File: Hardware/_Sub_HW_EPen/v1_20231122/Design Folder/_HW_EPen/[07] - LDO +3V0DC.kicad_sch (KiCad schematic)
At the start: 6 parts, among them U701 MIC5365-3.0YC5-TR

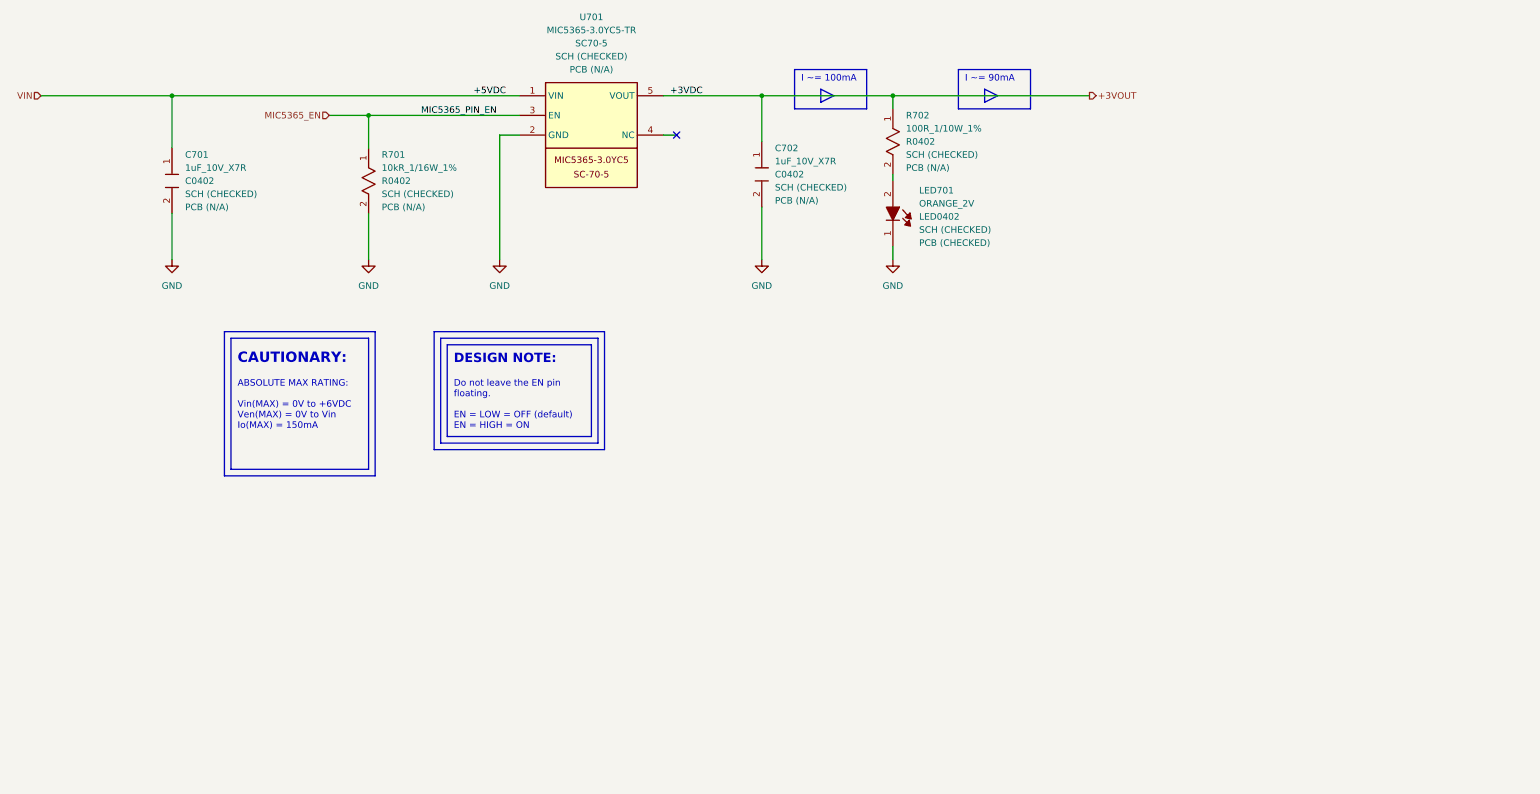
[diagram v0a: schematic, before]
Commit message: Updating file templates and structures...
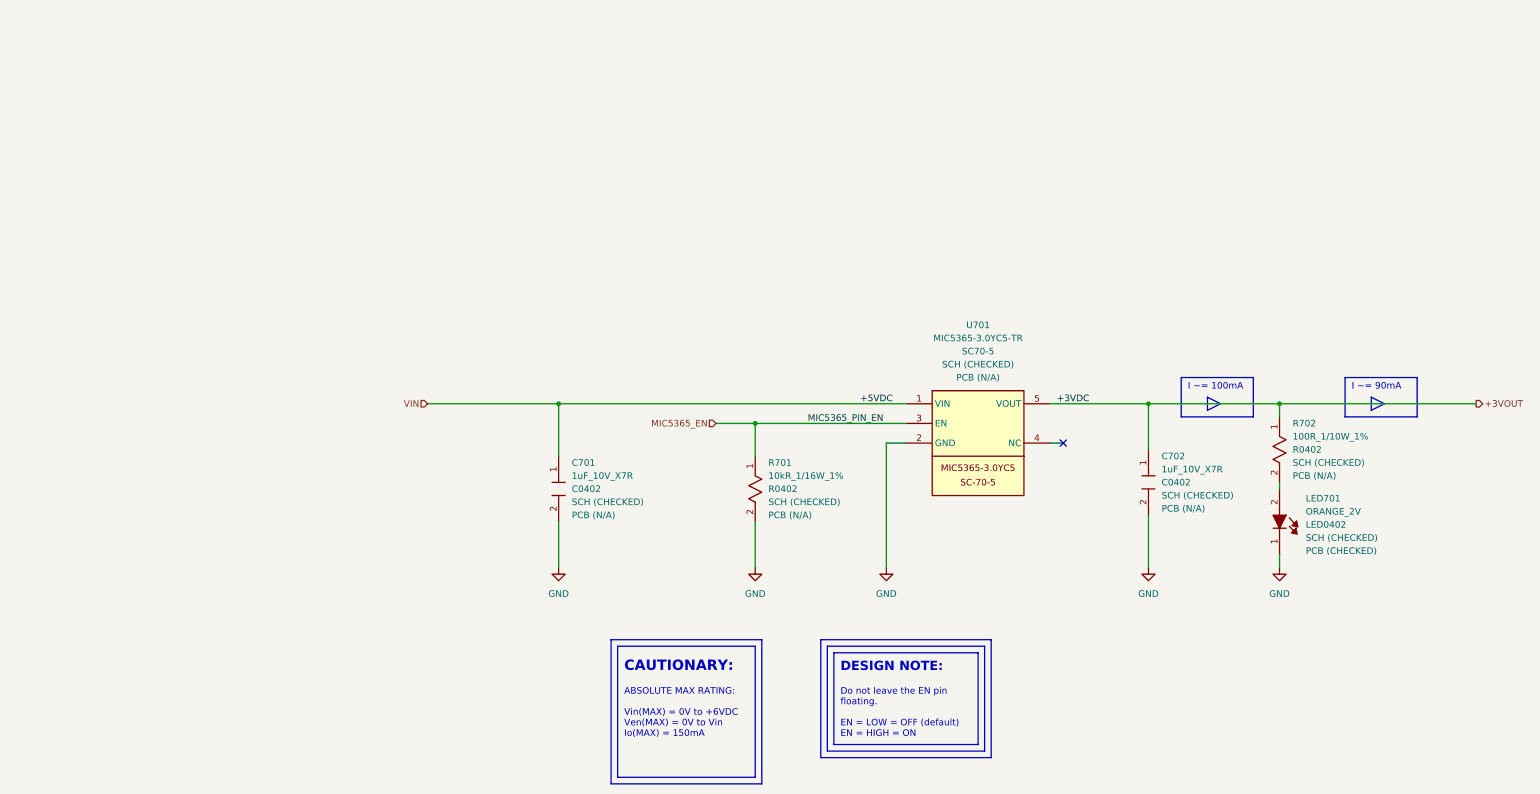
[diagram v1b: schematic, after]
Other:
- moved on the sheet: C701, C702, LED701, R701, R702, U701

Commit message: Updating Hardware File structures
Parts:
- C701, C702: Manufacturer (none) -> Murata Electronics; Part Number GRM155Z71A105KE01D -> (none); Part Number (Manufacturer) (none) -> GRM155Z71A105KE01D; Part Number (Vendor) (none) -> 490-GRM155Z71A105KE01DTR-ND; Vendor (none) -> Digikey
- LED701: Manufacturer (none) -> Harvatek Corporation; Part Number B2841UD--20D000614U1930 -> (none); Part Number (Manufacturer) (none) -> B2841UD--20D000614U1930; Part Number (Vendor) (none) -> 3147-B2841UD--20D000614U1930TR-ND; Vendor (none) -> Digikey
- R701: Manufacturer (none) -> Bourns Inc.; Part Number CR0402-FX-1002GLF -> (none); Part Number (Manufacturer) (none) -> CR0402-FX-1002GLF; Part Number (Vendor) (none) -> CR0402-FX-1002GLFTR-ND; Vendor (none) -> Digikey
- R702: Manufacturer (none) -> KOA Speer Electronics, Inc.; Part Number RK73H1ETTP1000F -> (none); Part Number (Manufacturer) (none) -> RK73H1ETTP1000F; Part Number (Vendor) (none) -> 2019-RK73H1ETTP1000FTR-ND; Vendor (none) -> Digikey
- U701: Manufacturer (none) -> Microchip Technology; Part Number MIC5365-3.0YC5-TR -> (none); Part Number (Manufacturer) (none) -> MIC5365-3.0YC5-TR; Part Number (Vendor) (none) -> 576-3191-2-ND; Vendor (none) -> Digikey
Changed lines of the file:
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@@
   (title_block
     (title "_HW_EPen")
-    (date "2023-11-28")
+    (date "2023/11/28")
     (rev "v1.0")
     (company "mend0z0")
     (comment 1 "v1.0")
     (comment 2 "CHECKED")
-    (comment 4 "_BOM_EPen.html")
-    (comment 5 "_HW_EPen.pcb")
+    (comment 3 "Siavash Taher Parvar")
+    (comment 4 "_BOM_EPen.csv")
+    (comment 5 "_HW_EPen.kicad_pcb")
     (comment 6 "_GBR_EPen.zip")
     (comment 7 "_BOM_EPen.html")
@@
       (effects (font (size 1.27 1.27)) (justify left) hide)
     )
-    (property "Part Number" "GRM155Z71A105KE01D" (at 220.98 191.77 0)
-      (effects (font (size 1.27 1.27)) (justify left) hide)
-    )
     (property "Link" "https://www.digikey.ca/en/products/detail/murata-electronics/GRM155Z71A105KE01D/13905035" (at 213.36 191.77 0)
       (effects (font (size 1.27 1.27)) (justify left) hide)
@@
       (effects (font (size 1.27 1.27)) (justify left))
     )
+    (property "Part Number (Vendor)" "490-GRM155Z71A105KE01DTR-ND" (at 201.93 189.23 0)
+      (effects (font (size 1.27 1.27)) hide)
+    )
+    (property "Part Number (Manufacturer)" "GRM155Z71A105KE01D" (at 223.52 191.77 0)
+      (effects (font (size 1.27 1.27)) (justify left) hide)
+    )
+    (property "Manufacturer" "Murata Electronics" (at 226.06 191.77 0)
+      (effects (font (size 1.27 1.27)) (justify left) hide)
+    )
+    (property "Vendor" "Digikey" (at 228.6 191.77 0)
+      (effects (font (size 1.27 1.27)) (justify left) hide)
+    )
     (pin "2")
     (pin "1")
@@
       (effects (font (size 1.27 1.27)) (justify left) hide)
     )
-    (property "Part Number" "RK73H1ETTP1000F" (at 360.68 184.15 0)
-      (effects (font (size 1.27 1.27)) (justify left) hide)
-    )
     (property "Link" "https://www.digikey.ca/en/products/detail/koa-speer-electronics-inc/RK73H1ETTP1000F/9844157" (at 353.06 184.15 0)
       (effects (font (size 1.27 1.27)) (justify left) hide)
@@
       (effects (font (size 1.27 1.27)) (justify left))
     )
+    (property "Part Number (Vendor)" "2019-RK73H1ETTP1000FTR-ND" (at 341.63 181.61 0)
+      (effects (font (size 1.27 1.27)) hide)
+    )
+    (property "Part Number (Manufacturer)" "RK73H1ETTP1000F" (at 363.22 184.15 0)
+      (effects (font (size 1.27 1.27)) (justify left) hide)
+    )
+    (property "Manufacturer" "KOA Speer Electronics, Inc." (at 365.76 184.15 0)
+      (effects (font (size 1.27 1.27)) (justify left) hide)
+    )
+    (property "Vendor" "Digikey" (at 368.3 184.15 0)
+      (effects (font (size 1.27 1.27)) (justify left) hide)
+    )
     (pin "1")
     (pin "2")
@@
       (effects (font (size 1.27 1.27)) (justify left) hide)
     )
-    (property "Part Number" "CR0402-FX-1002GLF" (at 259.08 191.77 0)
-      (effects (font (size 1.27 1.27)) (justify left) hide)
-    )
     (property "Link" "https://www.digikey.ca/en/products/detail/bourns-inc/CR0402-FX-1002GLF/3593192" (at 251.46 191.77 0)
       (effects (font (size 1.27 1.27)) (justify left) hide)
@@
       (effects (font (size 1.27 1.27)) (justify left))
     )
+    (property "Part Number (Vendor)" "CR0402-FX-1002GLFTR-ND" (at 240.03 189.23 0)
+      (effects (font (size 1.27 1.27)) hide)
+    )
+    (property "Part Number (Manufacturer)" "CR0402-FX-1002GLF" (at 261.62 191.77 0)
+      (effects (font (size 1.27 1.27)) (justify left) hide)
+    )
+    (property "Manufacturer" "Bourns Inc." (at 264.16 191.77 0)
+      (effects (font (size 1.27 1.27)) (justify left) hide)
+    )
+    (property "Vendor" "Digikey" (at 266.7 191.77 0)
+      (effects (font (size 1.27 1.27)) (justify left) hide)
+    )
     (pin "1")
     (pin "2")
@@
       (effects (font (size 1.27 1.27)) (justify left) hide)
     )
-    (property "Part Number" "B2841UD--20D000614U1930" (at 363.22 200.66 0)
-      (effects (font (size 1.27 1.27)) (justify left) hide)
-    )
     (property "Link" "https://www.digikey.ca/en/products/detail/harvatek-corporation/B2841UD-20D000614U1930/16729512" (at 355.6 200.66 0)
       (effects (font (size 1.27 1.27)) (justify left) hide)
@@
       (effects (font (size 1.27 1.27)) (justify left))
     )
+    (property "Part Number (Vendor)" "3147-B2841UD--20D000614U1930TR-ND" (at 341.63 195.58 0)
+      (effects (font (size 1.27 1.27)) hide)
+    )
+    (property "Part Number (Manufacturer)" "B2841UD--20D000614U1930" (at 365.76 200.66 0)
+      (effects (font (size 1.27 1.27)) (justify left) hide)
+    )
+    (property "Manufacturer" "Harvatek Corporation" (at 368.3 200.66 0)
+      (effects (font (size 1.27 1.27)) (justify left) hide)
+    )
+    (property "Vendor" "Digikey" (at 370.84 200.66 0)
+      (effects (font (size 1.27 1.27)) (justify left) hide)
+    )
     (pin "2")
     (pin "1")
@@
       (effects (font (size 1.27 1.27)) (justify left) hide)
     )
-    (property "Part Number" "GRM155Z71A105KE01D" (at 335.28 190.5 0)
-      (effects (font (size 1.27 1.27)) (justify left) hide)
-    )
     (property "Link" "https://www.digikey.ca/en/products/detail/murata-electronics/GRM155Z71A105KE01D/13905035" (at 327.66 190.5 0)
       (effects (font (size 1.27 1.27)) (justify left) hide)
@@
       (effects (font (size 1.27 1.27)) (justify left))
     )
+    (property "Part Number (Vendor)" "490-GRM155Z71A105KE01DTR-ND" (at 316.23 187.96 0)
+      (effects (font (size 1.27 1.27)) hide)
+    )
+    (property "Part Number (Manufacturer)" "GRM155Z71A105KE01D" (at 337.82 190.5 0)
+      (effects (font (size 1.27 1.27)) (justify left) hide)
+    )
+    (property "Manufacturer" "Murata Electronics" (at 340.36 190.5 0)
+      (effects (font (size 1.27 1.27)) (justify left) hide)
+    )
+    (property "Vendor" "Digikey" (at 342.9 190.5 0)
+      (effects (font (size 1.27 1.27)) (justify left) hide)
+    )
     (pin "2")
     (pin "1")
@@
       (effects (font (size 1.27 1.27)) (justify left) hide)
     )
-    (property "Part Number" "MIC5365-3.0YC5-TR" (at 276.86 157.48 0)
-      (effects (font (size 1.27 1.27)) (justify left) hide)
-    )
     (property "Link" "https://www.digikey.ca/en/products/detail/microchip-technology/MIC5365-3-0YC5-TR/1868092" (at 276.86 165.1 0)
       (effects (font (size 1.27 1.27)) (justify left) hide)
@@
       (effects (font (size 1.27 1.27)))
     )
-    (pin "1")
+    (property "Part Number (Vendor)" "576-3191-2-ND" (at 274.32 176.53 0)
+      (effects (font (size 1.27 1.27)) hide)
+    )
+    (property "Part Number (Manufacturer)" "MIC5365-3.0YC5-TR" (at 276.86 154.94 0)
+      (effects (font (size 1.27 1.27)) (justify left) hide)
+    )
+    (property "Manufacturer" "Microchip Technology" (at 276.86 152.4 0)
+      (effects (font (size 1.27 1.27)) (justify left) hide)
+    )
+    (property "Vendor" "Digikey" (at 276.86 149.86 0)
+      (effects (font (size 1.27 1.27)) (justify left) hide)
+    )
+    (pin "1")
